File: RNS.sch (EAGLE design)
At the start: 12 parts

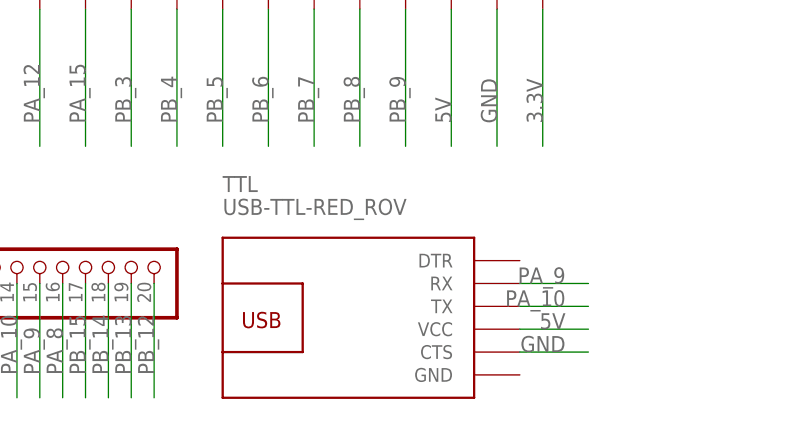
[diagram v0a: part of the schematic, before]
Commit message: Add files via upload
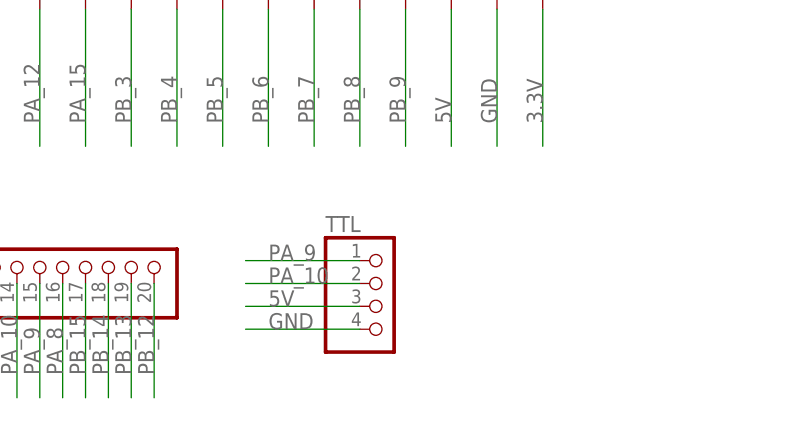
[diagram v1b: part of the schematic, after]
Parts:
- TTL: value USB-TTL-RED_ROV -> (none); device MIA_LIBRARY-2-2-2:USB-TTL-RED_ROV -> MIA_LIBRARY-2-2-2:PINHD-1X4
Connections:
- net 5V: now also TTL.3; no longer TTL.VCC
- net GND: now also TTL.4; no longer TTL.CTS
- net PA_10: now also TTL.2; no longer TTL.TX
- net PA_9: now also TTL.1; no longer TTL.RX
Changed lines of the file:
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@@
 <part name="POWER_BASE" library="MIA_LIBRARY-2-2-2" deviceset="PINHD-2_DATA" device="" package3d_urn="urn:adsk.eagle:package:15814197/4"/>
 <part name="CYTRON" library="MIA_LIBRARY-2-2-2" deviceset="PINHD-3_DATA" device="" package3d_urn="urn:adsk.eagle:package:15814198/11"/>
-<part name="TTL" library="MIA_LIBRARY-2-2-2" deviceset="USB-TTL-RED_ROV" device="" package3d_urn="urn:adsk.eagle:package:15814141/1"/>
 <part name="VOLTAGE_REGULATOR" library="MIA_LIBRARY-2-2-2" deviceset="78XXS" device="" package3d_urn="urn:adsk.eagle:package:15814050/2"/>
 <part name="IMU" library="MIA_LIBRARY-2-2-2" deviceset="IMU_ROBOCON_GY521" device="" package3d_urn="urn:adsk.eagle:package:15814143/2"/>
@@
 <part name="LED" library="led" library_urn="urn:adsk.eagle:library:259" deviceset="LED" device="5MM" package3d_urn="urn:adsk.eagle:package:15799/2"/>
 <part name="RESISTOR" library="rcl" library_urn="urn:adsk.eagle:library:334" deviceset="R-EU_" device="0207/12" package3d_urn="urn:adsk.eagle:package:23489/1"/>
+<part name="TTL" library="MIA_LIBRARY-2-2-2" deviceset="PINHD-1X4" device="" package3d_urn="urn:adsk.eagle:package:22407/2"/>
 </parts>
 <sheets>
@@
 <attribute name="VALUE" x="143.51" y="88.9" size="1.778" layer="96"/>
 </instance>
-<instance part="TTL" gate="G$1" x="55.88" y="0" smashed="yes" grouprefs="UC">
-<attribute name="NAME" x="43.18" y="15.24" size="1.778" layer="95"/>
-<attribute name="VALUE" x="43.18" y="12.7" size="1.778" layer="96"/>
-</instance>
 <instance part="VOLTAGE_REGULATOR" gate="1" x="-76.2" y="73.66" smashed="yes" grouprefs="POWER_AND_INDICATION">
 <attribute name="NAME" x="-73.66" y="66.04" size="1.778" layer="95"/>
@@
 <attribute name="VALUE" x="-54.61" y="54.102" size="1.778" layer="96" rot="R180"/>
 </instance>
+<instance part="TTL" gate="A" x="60.96" y="2.54" smashed="yes" grouprefs="UC">
+<attribute name="NAME" x="54.61" y="10.795" size="1.778" layer="95"/>
+<attribute name="VALUE" x="54.61" y="-5.08" size="1.778" layer="96"/>
+</instance>
 </instances>
 <busses>
@@
 </segment>
 <segment>
-<pinref part="TTL" gate="G$1" pin="RX"/>
-<wire x1="76.2" y1="5.08" x2="83.82" y2="5.08" width="0.1524" layer="91" grouprefs="UC"/>
-<label x="81.28" y="5.08" size="1.778" layer="95" align="bottom-right" grouprefs="UC"/>
-</segment>
-<segment>
 <pinref part="STM_PINS1" gate="A" pin="15"/>
 <wire x1="22.86" y1="5.08" x2="22.86" y2="-7.62" width="0.1524" layer="91" grouprefs="UC"/>
 <label x="22.86" y="-5.08" size="1.778" layer="95" rot="R90" grouprefs="UC"/>
 </segment>
+<segment>
+<pinref part="TTL" gate="A" pin="1"/>
+<wire x1="58.42" y1="7.62" x2="45.72" y2="7.62" width="0.1524" layer="91"/>
+<label x="48.26" y="7.62" size="1.778" layer="95"/>
+</segment>
 </net>
 <net name="PA_10" class="0">
@@
 </segment>
 <segment>
-<pinref part="TTL" gate="G$1" pin="TX"/>
-<wire x1="76.2" y1="2.54" x2="83.82" y2="2.54" width="0.1524" layer="91" grouprefs="UC"/>
-<label x="81.28" y="2.54" size="1.778" layer="95" align="bottom-right" grouprefs="UC"/>
-</segment>
-<segment>
 <pinref part="STM_PINS1" gate="A" pin="14"/>
 <wire x1="20.32" y1="5.08" x2="20.32" y2="-7.62" width="0.1524" layer="91" grouprefs="UC"/>
 <label x="20.32" y="-5.08" size="1.778" layer="95" rot="R90" grouprefs="UC"/>
 </segment>
+<segment>
+<pinref part="TTL" gate="A" pin="2"/>
+<wire x1="58.42" y1="5.08" x2="45.72" y2="5.08" width="0.1524" layer="91"/>
+<label x="48.26" y="5.08" size="1.778" layer="95"/>
+</segment>
 </net>
 <net name="PA_11" class="0">
@@
 </segment>
 <segment>
-<pinref part="TTL" gate="G$1" pin="VCC"/>
-<wire x1="76.2" y1="0" x2="83.82" y2="0" width="0.1524" layer="91" grouprefs="UC"/>
-<label x="81.28" y="0" size="1.778" layer="95" align="bottom-right" grouprefs="UC"/>
-</segment>
-<segment>
 <pinref part="ENCODER" gate="G$1" pin="VCC"/>
 <wire x1="144.78" y1="17.78" x2="132.08" y2="17.78" width="0.1524" layer="91" grouprefs="MOTOR_AND_SENSORS"/>
@@
 <label x="-81.28" y="63.5" size="1.778" layer="95" rot="R90" align="bottom-right"/>
 </segment>
+<segment>
+<pinref part="TTL" gate="A" pin="3"/>
+<wire x1="58.42" y1="2.54" x2="45.72" y2="2.54" width="0.1524" layer="91"/>
+<label x="48.26" y="2.54" size="1.778" layer="95"/>
+</segment>
 </net>
 <net name="3.3V" class="0">
@@
 </segment>
 <segment>
-<pinref part="TTL" gate="G$1" pin="CTS"/>
-<wire x1="76.2" y1="-2.54" x2="83.82" y2="-2.54" width="0.1524" layer="91" grouprefs="UC"/>
-<label x="81.28" y="-2.54" size="1.778" layer="95" align="bottom-right" grouprefs="UC"/>
-</segment>
-<segment>
 <pinref part="CYTRON" gate="A" pin="3"/>
 <wire x1="147.32" y1="93.98" x2="134.62" y2="93.98" width="0.1524" layer="91" grouprefs="MOTOR_AND_SENSORS"/>
@@
 <label x="-43.18" y="50.8" size="1.778" layer="95" align="bottom-right"/>
 </segment>
-</net>
+<segment>
+<pinref part="TTL" gate="A" pin="4"/>
+<wire x1="58.42" y1="0" x2="45.72" y2="0" width="0.1524" layer="91"/>
+<label x="48.26" y="0" size="1.778" layer="95"/>
+</segment>
+</net>
